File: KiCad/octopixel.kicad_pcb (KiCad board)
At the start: 2 copper layers, 25.8 x 35.5 mm, 8 parts, among them J2 RBG PB3, J3 RBG PB4, J4 RBG PB5, J5 RBG_PB3, J6 Octopus SPI3, U1 CD4050BE

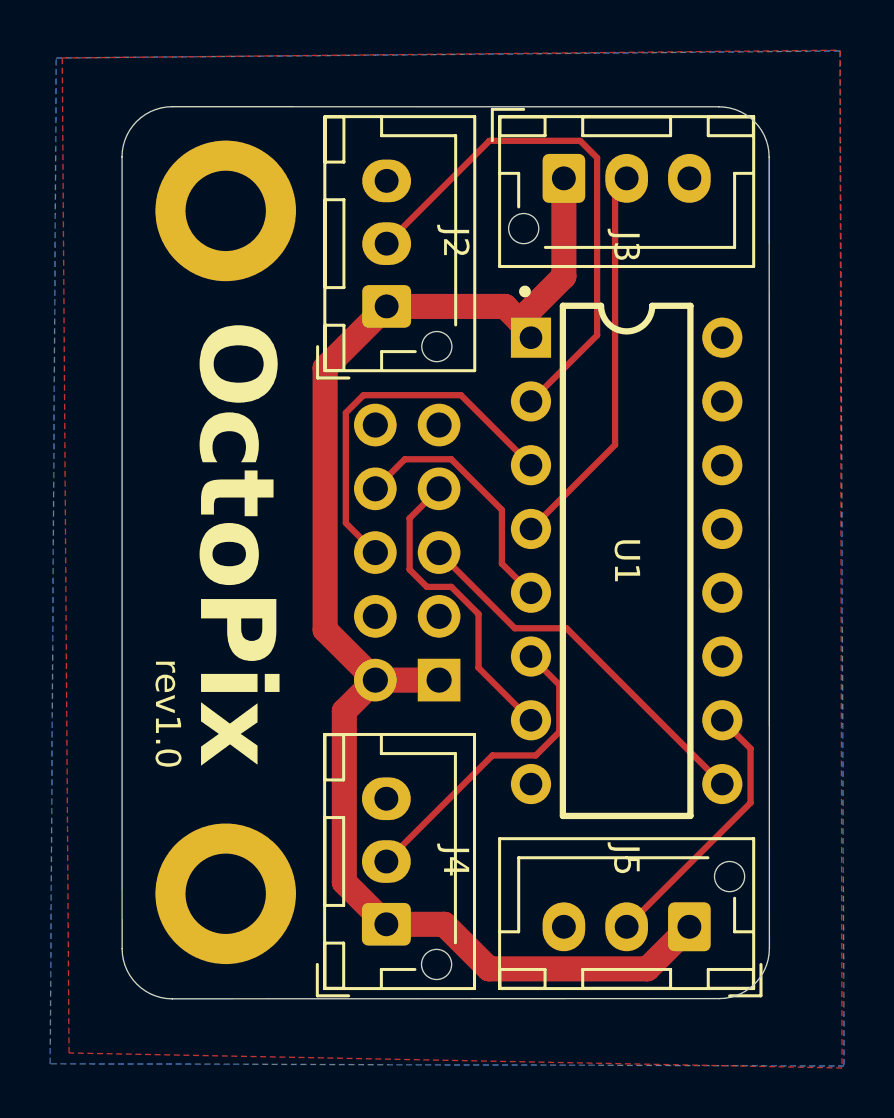
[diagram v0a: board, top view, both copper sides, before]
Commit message: Intial commit for SMD version
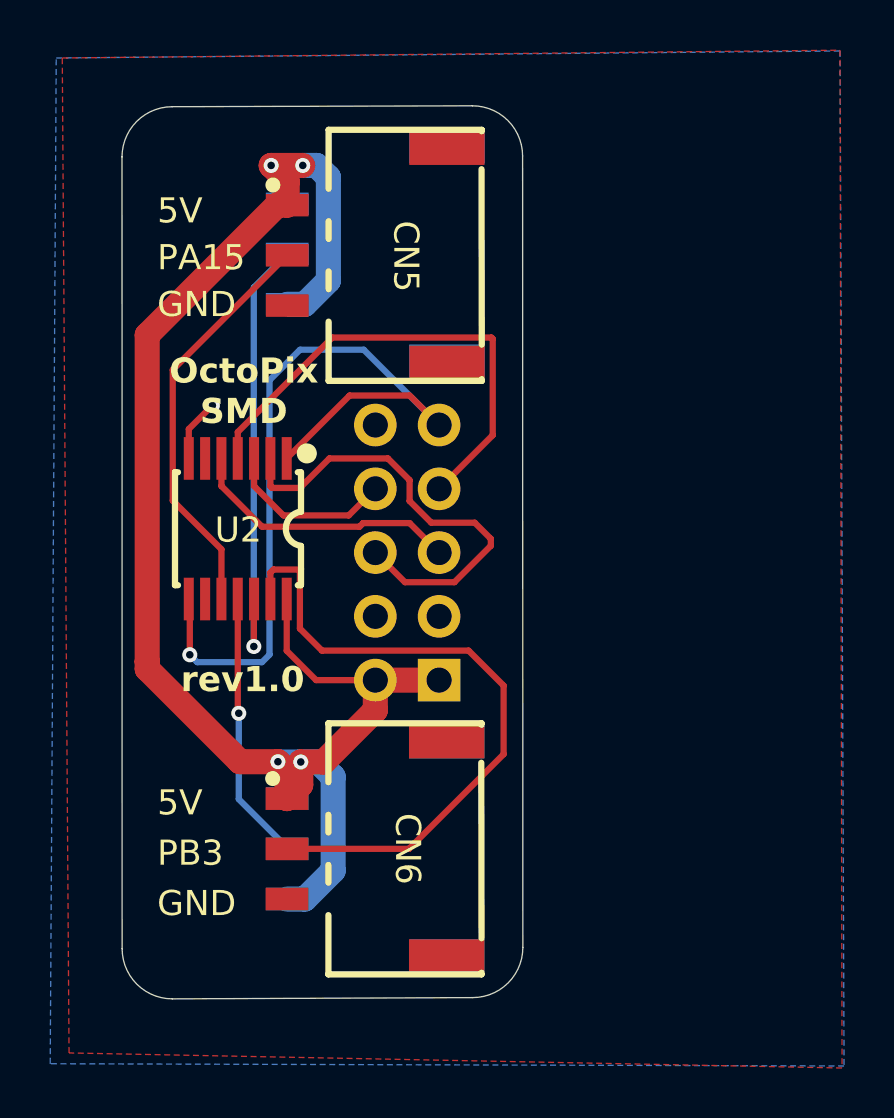
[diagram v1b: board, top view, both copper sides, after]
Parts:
- removed H1, H2: MountingHole, MountingHole:MountingHole_3.2mm_M3_DIN965_Pad
- removed J2: RBG PB3, Connector_JST:JST_XH_B3B-XH-AM_1x03_P2.50mm_Vertical
- removed J3: RBG PB4, Connector_JST:JST_XH_B3B-XH-AM_1x03_P2.50mm_Vertical
- removed J4: RBG PB5, Connector_JST:JST_XH_B3B-XH-AM_1x03_P2.50mm_Vertical
- removed J5: RBG_PB3, Connector_JST:JST_XH_B3B-XH-AM_1x03_P2.50mm_Vertical
- removed U1: CD4050BE, easyeda:DIP-16_L20.3-W10.2-P2.54-LS10.2-BL
- added CN5: PH2.0-3PWB Horizontal, easyeda:CONN-TH_PH-3PWB, F.Cu at (94.6, 37.4)
- added CN6: PH2.0-3PWB Horizontal, easyeda:CONN-TH_PH-3PWB, F.Cu at (94.6, 61.1)
- added CN7: PH2.0-3PWB Horizontal, easyeda:CONN-TH_PH-3PWB, B.Cu at (94.6, 37.4)
- added CN8: PH2.0-3PWB Horizontal, easyeda:CONN-TH_PH-3PWB, B.Cu at (94.6, 61.1)
- added U2: TXS0104EPWR, easyeda:TSSOP-14_L5.0-W4.4-P0.65-LS6.4-BL, F.Cu at (89.5, 48.3)
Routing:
- net +3V3: track 0.00 -> 32.7 mm, vias 0 -> 1
- net +5V: track 55.6 -> 63.7 mm, vias 0 -> 4
- net PB5: track 12.3 -> 19.6 mm
- net PA15_{5V}: track 10.7 -> 16.4 mm
- net PB3_{5V}: track 21.2 -> 26.6 mm
- net PA15: track 15.1 -> 11.0 mm
- net PB3: track 14.9 -> 18.2 mm
- net PB4: track 10.1 -> 6.85 mm
- net PB4_{5V}: track 15.3 -> 18.1 mm, vias 0 -> 1
- net GND: track 0.00 -> 2.50 mm, vias 0 -> 1
- net PB5_{5V}: track 12.5 -> 10.8 mm, vias 0 -> 1
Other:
- board size 25.8 x 35.5 mm -> 16 x 35.6 mm
- board text added: "OctoPix SMD"
- board text added: "PA15"
- board text removed: "OctoPix"
- board text removed: "PB15"
